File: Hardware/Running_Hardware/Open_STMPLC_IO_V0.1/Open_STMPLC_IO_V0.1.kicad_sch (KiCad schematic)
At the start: 73 parts, among them J1 Screw_Terminal_01x02, J2 Screw_Terminal_01x02, J3 Screw_Terminal_01x02, J4 Screw_Terminal_01x02, J5 Screw_Terminal_01x04, Q1 SUD50P06, Q2 AO3400A, SW1 SW_SPDT, SW2 SW_SPDT, SW3 SW_DIP_x02, SW4 SW_SPDT, U10 MAX31865xTP, U11 MAX31856, U12 6N137, U3 TPS1H200A, U7 TPS26600PWP, U8 UCC23513

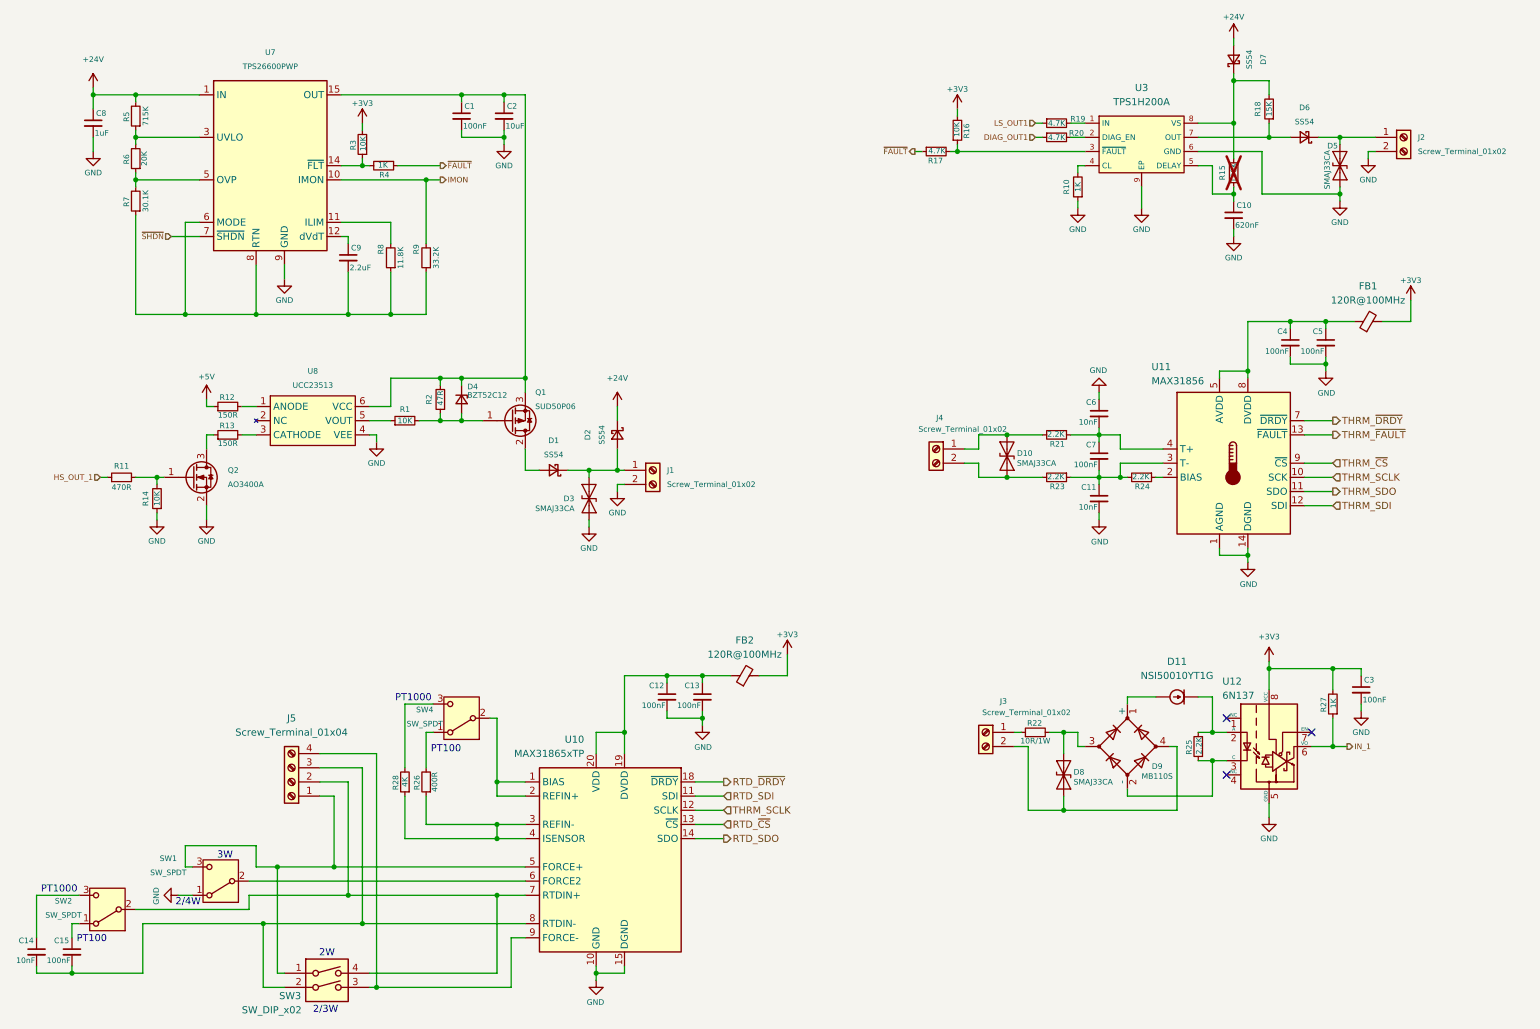
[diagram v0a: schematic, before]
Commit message: IO board changes
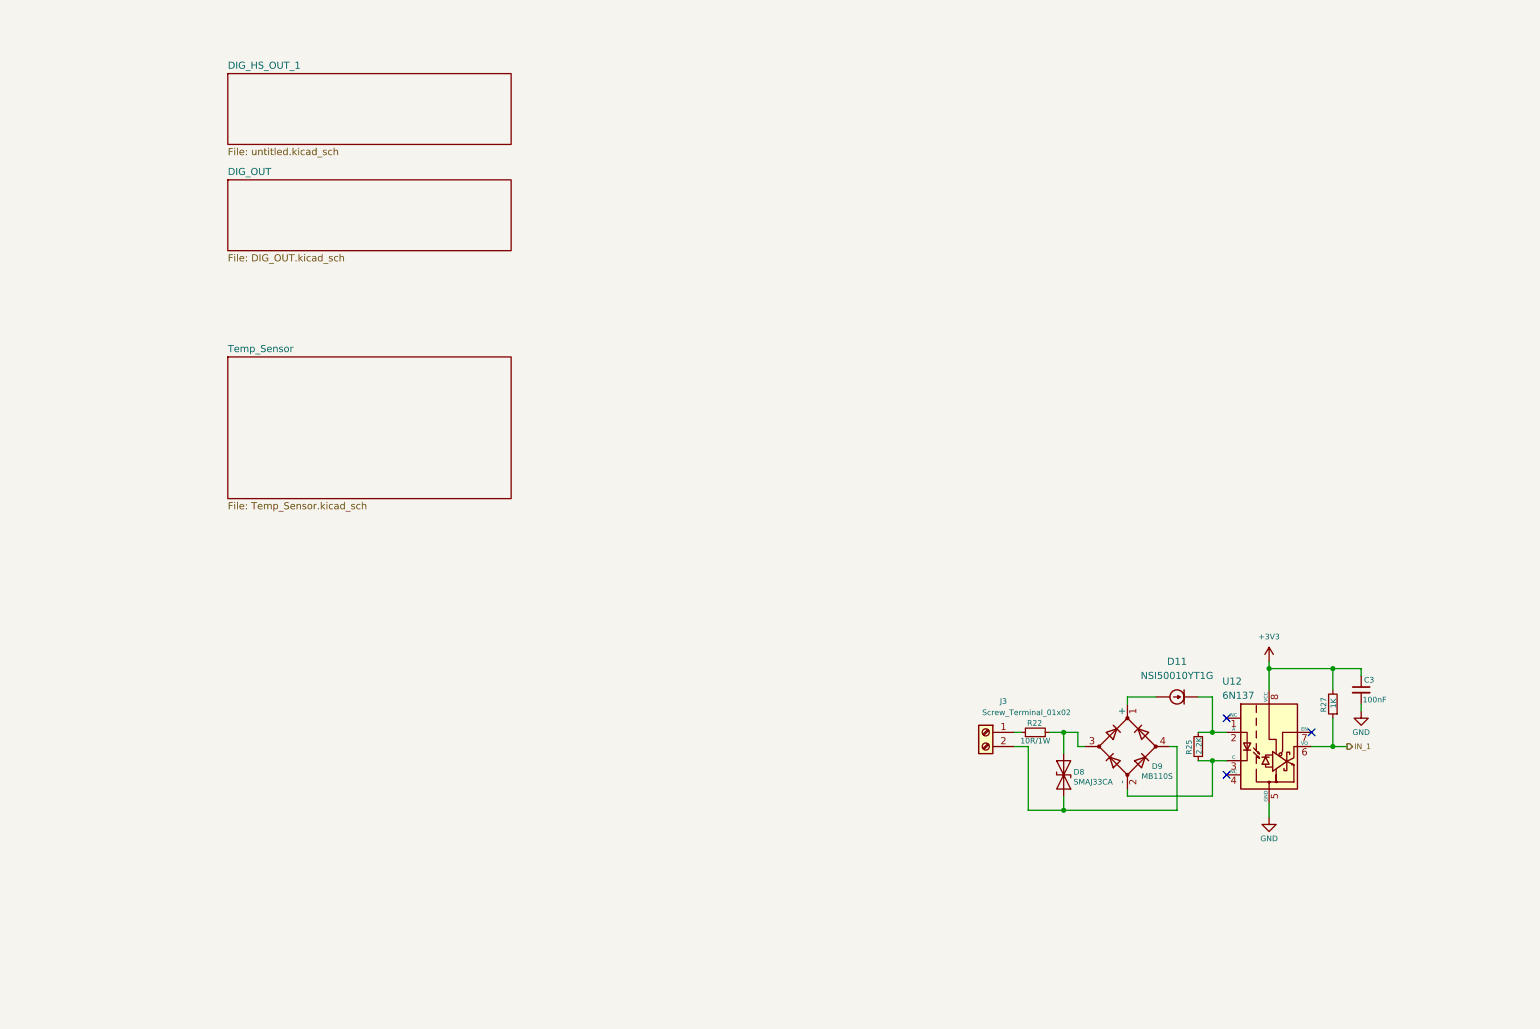
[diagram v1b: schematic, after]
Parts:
- removed C1: 100nF, symbol Device:C_Small
- removed C10: 620nF, symbol Device:C_Small
- removed C11, C14, C6: 10nF, Capacitor_SMD:C_0603_1608Metric_Pad1.08x0.95mm_HandSolder, symbol Device:C_Small
- removed C12, C13, C15, C4, C5, C7: 100nF, Capacitor_SMD:C_0603_1608Metric_Pad1.08x0.95mm_HandSolder, symbol Device:C_Small
- removed C2: 10uF, symbol Device:C_Small
- removed C8: 1uF, symbol Device:C_Small
- removed C9: 2.2uF, symbol Device:C_Small
- removed D1, D2, D6, D7: SS54, symbol Device:D_Schottky_Small
- removed D10, D3, D5: SMAJ33CA, Diode_SMD:D_SMA, symbol Diode:SMAJ33CA
- removed D4: BZT52C12, symbol Device:D_Zener_Small
- removed FB1, FB2: 120R@100MHz, symbol Device:FerriteBead_Small
- removed J1, J2, J4: Screw_Terminal_01x02, symbol Connector:Screw_Terminal_01x02
- removed J5: Screw_Terminal_01x04, symbol Connector:Screw_Terminal_01x04
- removed Q1: SUD50P06, Package_TO_SOT_SMD:TO-252-3_TabPin2, symbol Transistor_FET:Q_PMOS_GDS
- removed Q2: AO3400A, Package_TO_SOT_SMD:SOT-23, symbol Transistor_FET:AO3400A
- removed R1, R14: 10K, symbol Device:R_Small
- removed R10: 1K, symbol Device:R_Small
- removed R11: 470R, symbol Device:R_Small
- removed R12, R13: 150R, Resistor_SMD:R_0603_1608Metric_Pad0.98x0.95mm_HandSolder, symbol Device:R_Small
- removed R15: 100K, symbol Device:R_Small
- removed R16, R3: 10K, Resistor_SMD:R_0603_1608Metric_Pad0.98x0.95mm_HandSolder, symbol Device:R_Small
- removed R17, R19, R20: 4.7K, Resistor_SMD:R_0603_1608Metric_Pad0.98x0.95mm_HandSolder, symbol Device:R_Small
- removed R18: 15K, symbol Device:R_Small
- removed R2: 47R, symbol Device:R_Small
- removed R21, R23, R24: 2.2K, Resistor_SMD:R_0603_1608Metric_Pad0.98x0.95mm_HandSolder, symbol Device:R_Small
- removed R26: 400R, Resistor_SMD:R_0603_1608Metric_Pad0.98x0.95mm_HandSolder, symbol Device:R_Small
- removed R28: 4K, Resistor_SMD:R_0603_1608Metric_Pad0.98x0.95mm_HandSolder, symbol Device:R_Small
- removed R4: 1K, Resistor_SMD:R_0603_1608Metric_Pad0.98x0.95mm_HandSolder, symbol Device:R_Small
- removed R5: 715K, Resistor_SMD:R_0603_1608Metric_Pad0.98x0.95mm_HandSolder, symbol Device:R_Small
- removed R6: 20K, Resistor_SMD:R_0603_1608Metric_Pad0.98x0.95mm_HandSolder, symbol Device:R_Small
- removed R7: 30.1K, Resistor_SMD:R_0603_1608Metric_Pad0.98x0.95mm_HandSolder, symbol Device:R_Small
- removed R8: 11.8K, Resistor_SMD:R_0603_1608Metric_Pad0.98x0.95mm_HandSolder, symbol Device:R_Small
- removed R9: 33.2K, Resistor_SMD:R_0603_1608Metric_Pad0.98x0.95mm_HandSolder, symbol Device:R_Small
- removed SW1, SW2, SW4: SW_SPDT, symbol Switch:SW_SPDT
- removed SW3: SW_DIP_x02, symbol Switch:SW_DIP_x02
- removed U10: MAX31865xTP, Package_DFN_QFN:TQFN-20-1EP_5x5mm_P0.65mm_EP3.25x3.25mm, symbol Sensor_Temperature:MAX31865xTP
- removed U11: MAX31856, Package_SO:TSSOP-14_4.4x5mm_P0.65mm, symbol Sensor_Temperature:MAX31856
- removed U3: TPS1H200A, Package_SO:HVSSOP-8-1EP_3x3mm_P0.65mm_EP1.57x1.89mm_ThermalVias, symbol TPS1H200A:TPS1H200A
- removed U7: TPS26600PWP, Package_SO:HTSSOP-16-1EP_4.4x5mm_P0.65mm_EP3.4x5mm_Mask2.66x2.46mm_ThermalVias, symbol Power_Management:TPS26600PWP
- removed U8: UCC23513, Package_SO:SSO-6_6.8x4.6mm_P1.27mm_Clearance8mm, symbol UCC23153:UCC23513
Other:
- added sheet DIG_HS_OUT_1 (untitled.kicad_sch)
- added sheet DIG_OUT (DIG_OUT.kicad_sch)
- added sheet Temp_Sensor (Temp_Sensor.kicad_sch)
- note removed: "2/3W"
- note removed: "2/4W"
- note removed: "2W"
- note removed: "3W"
- note removed: "PT100"
- note removed: "PT1000"
